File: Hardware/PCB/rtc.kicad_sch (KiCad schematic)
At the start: 4 parts, among them U7 DS3232M

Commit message: fixed BOM, added some silkscreen, getting quote now
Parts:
- C21: DigiKey Link https://www.digikey.com/en/products/detail/samsung-electro-mechanics/CL10B105KP8NNNC/3887604 -> https://www.digikey.com/en/products/detail/samsung-electro-mechanics/CL10B105KO8NNNC/3886677; MPN CL10B105KP8NNNC -> CL10B105KO8NNNC
- C22: DigiKey Link (none) -> https://www.digikey.com/en/products/detail/samsung-electro-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; MPN GCM188R71H104KA57J -> CL10B104KO8NNNC; Manufacturer (none) -> Samsung Electro-Mechanics
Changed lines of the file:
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@@
 			)
 		)
-		(property "Description" "1 µF ±10% 10V Ceramic Capacitor X7R 0603 (1608 Metric)"
+		(property "Description" "1 µF ±10% 16V Ceramic Capacitor X7R 0603 (1608 Metric)"
 			(at 133.35 36.83 0)
 			(effects
@@
 			)
 		)
-		(property "DigiKey Link" "https://www.digikey.com/en/products/detail/samsung-electro-mechanics/CL10B105KP8NNNC/3887604"
+		(property "DigiKey Link" "https://www.digikey.com/en/products/detail/samsung-electro-mechanics/CL10B105KO8NNNC/3886677"
 			(at 133.35 36.83 0)
 			(effects
@@
 			)
 		)
-		(property "MPN" "CL10B105KP8NNNC"
+		(property "MPN" "CL10B105KO8NNNC"
 			(at 133.35 36.83 0)
 			(effects
@@
 			)
 		)
-		(property "Description" "0.1 µF ±10% 50V Ceramic Capacitor X7R 0603 (1608 Metric)"
+		(property "Description" "0.1 µF ±10% 16V Ceramic Capacitor X7R 0603 (1608 Metric)"
 			(at 144.78 36.83 0)
 			(effects
@@
 			)
 		)
-		(property "MPN" "GCM188R71H104KA57J"
+		(property "MPN" "CL10B104KO8NNNC"
 			(at 144.78 36.83 0)
 			(effects
+				(font
+					(size 1.27 1.27)
+				)
+				(hide yes)
+			)
+		)
+		(property "DigiKey Link" "https://www.digikey.com/en/products/detail/samsung-electro-mechanics/CL10B104KO8NNNC/3886663"
+			(at 144.78 36.83 0)
+			(effects
+				(font
+					(size 1.27 1.27)
+				)
+				(hide yes)
+			)
+		)
+		(property "Manufacturer" "Samsung Electro-Mechanics"
+			(at 144.78 36.83 0)
+			(effects
+				(font
+					(size 1.27 1.27)
+				)
+				(hide yes)
+			)
+		)
+		(property "Mouser Link" ""
+			(at 144.78 36.83 0)
+			(effects

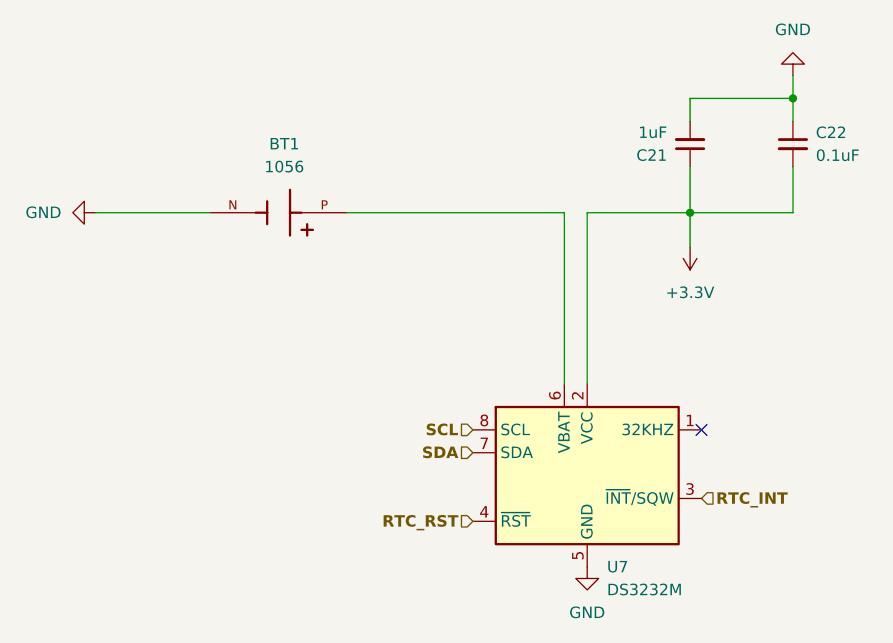
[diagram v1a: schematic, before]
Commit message: kinda pricey, I should try to make a smaller version using LCSC parts for cheaper solution
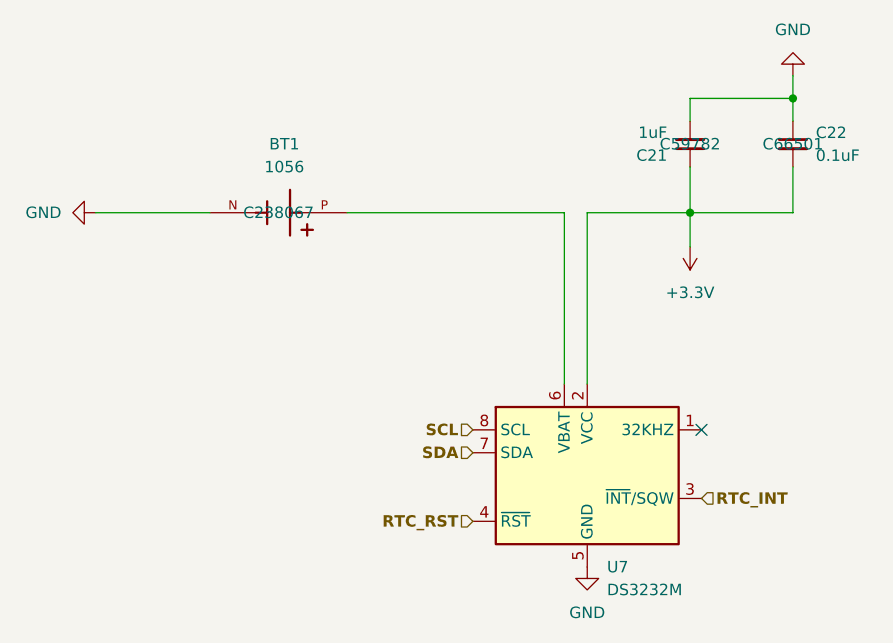
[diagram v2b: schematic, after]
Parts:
- BT1: LCSC (none) -> C238067
- C21: LCSC (none) -> C59782
- C22: LCSC (none) -> C66501
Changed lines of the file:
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@@
+			)
+		)
+		(property "LCSC" ""
+			(at 121.92 73.66 0)
+			(effects
+				(font
+					(size 1.27 1.27)
+				)
 			)
 		)
@@
 			)
 		)
+		(property "LCSC" "C59782"
+			(at 133.35 36.83 0)
+			(effects
+				(font
+					(size 1.27 1.27)
+				)
+			)
+		)
 		(pin "2"
 		)
@@
 			)
 		)
+		(property "LCSC" "C66501"
+			(at 144.78 36.83 0)
+			(effects
+				(font
+					(size 1.27 1.27)
+				)
+			)
+		)
 		(pin "1"
 		)
@@
 			)
 		)
+		(property "LCSC" "C238067"
+			(at 87.63 44.45 0)
+			(effects
+				(font
+					(size 1.27 1.27)
+				)
+			)
+		)

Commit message: done with this, placed order
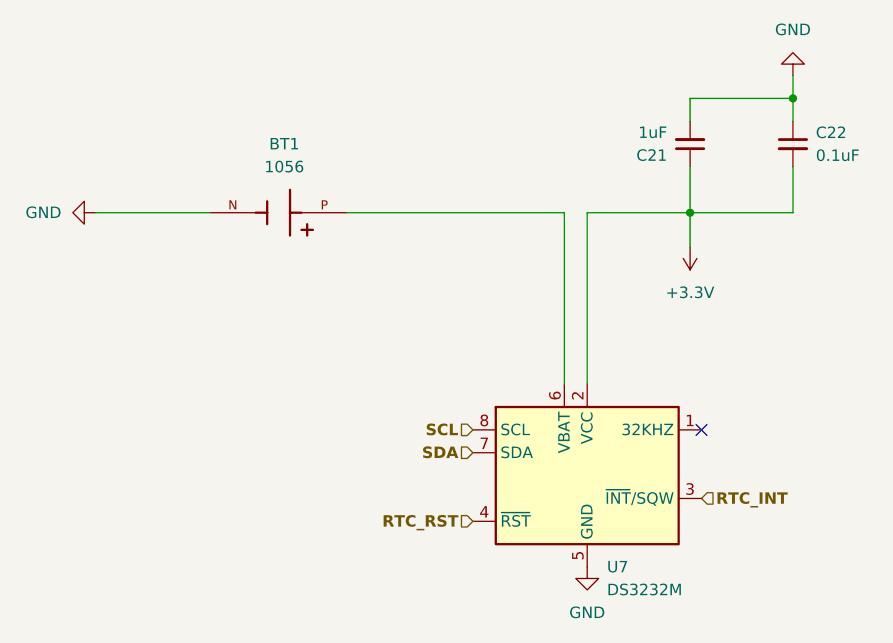
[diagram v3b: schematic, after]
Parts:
- BT1: LCSC C238067 -> (none)
- C21: LCSC C59782 -> (none)
- C22: LCSC C66501 -> (none)
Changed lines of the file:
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@@
-			)
-		)
-		(property "LCSC" ""
-			(at 121.92 73.66 0)
-			(effects
-				(font
-					(size 1.27 1.27)
-				)
 			)
 		)
@@
 			)
 		)
-		(property "LCSC" "C59782"
-			(at 133.35 36.83 0)
-			(effects
-				(font
-					(size 1.27 1.27)
-				)
-			)
-		)
 		(pin "2"
 		)
@@
 			)
 		)
-		(property "LCSC" "C66501"
-			(at 144.78 36.83 0)
-			(effects
-				(font
-					(size 1.27 1.27)
-				)
-			)
-		)
 		(pin "1"
 		)
@@
 			)
 		)
-		(property "LCSC" "C238067"
-			(at 87.63 44.45 0)
-			(effects
-				(font
-					(size 1.27 1.27)
-				)
-			)
-		)
